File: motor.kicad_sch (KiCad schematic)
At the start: 20 parts, among them J201 JST-SH, J202 JST-SH, J203 JST-SH, J204 JST-SH, U201 A4950E, U202 A4950E, U203 A4950E, U204 A4950E

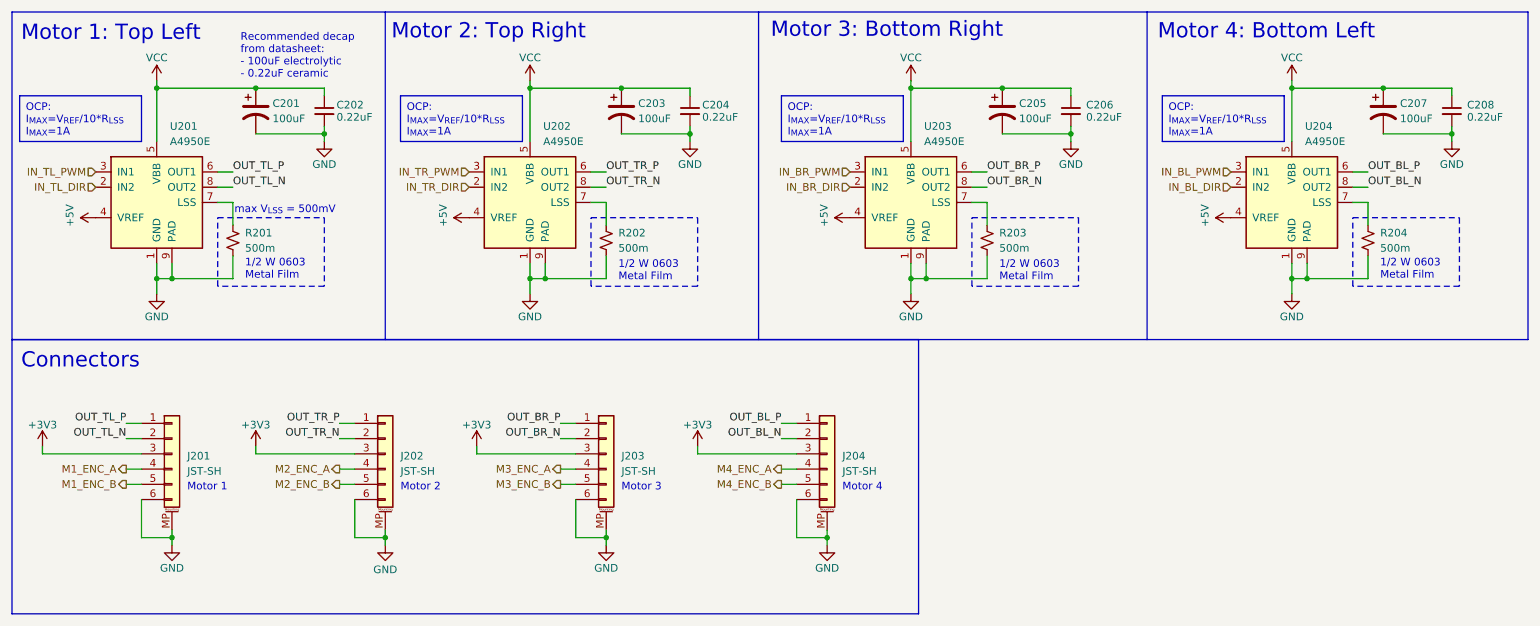
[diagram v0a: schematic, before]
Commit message: version 2 done
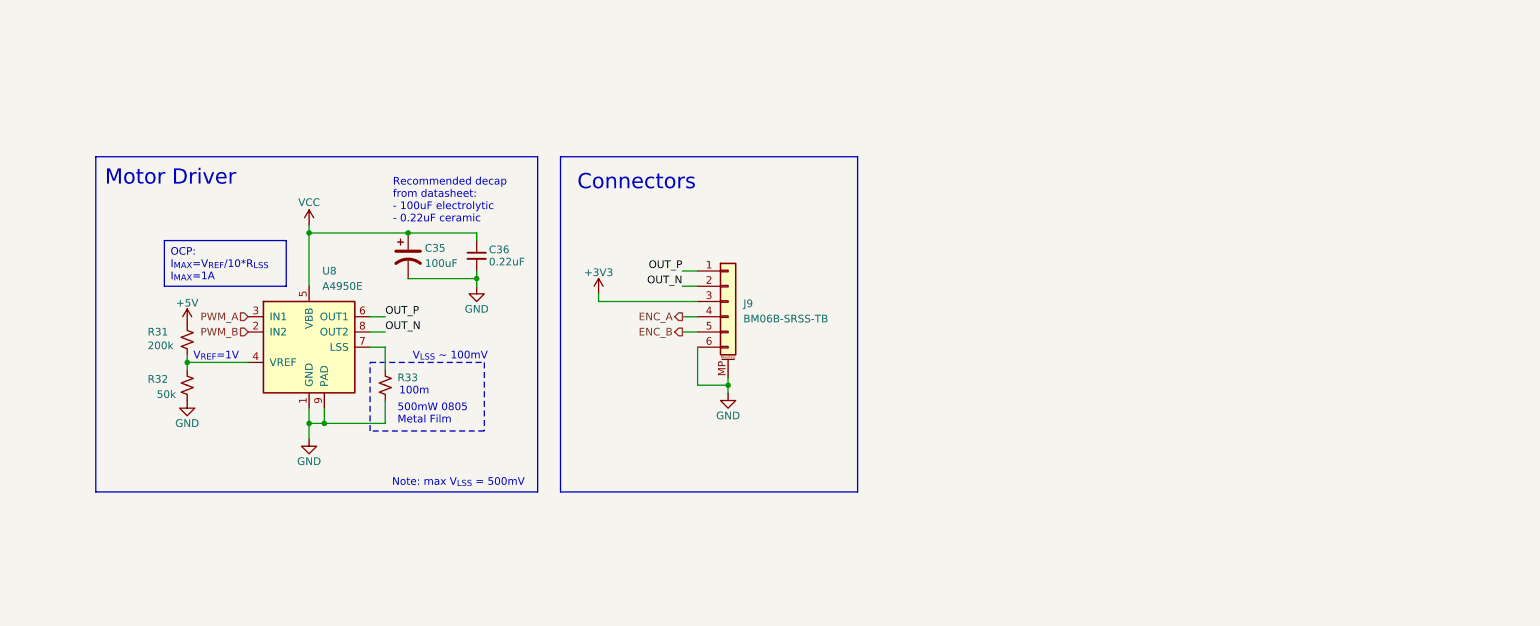
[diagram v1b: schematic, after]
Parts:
- removed C203, C205, C207: 100uF, Capacitor_SMD:CP_Elec_6.3x7.7, symbol Device:C_Polarized_US
- removed C204, C206, C208: 0.22uF, Capacitor_SMD:C_0603_1608Metric, symbol Device:C_Small
- removed J202, J203, J204: JST-SH, Connector_JST:JST_SH_SM06B-SRSS-TB_1x06-1MP_P1.00mm_Horizontal, symbol Connector_Generic_MountingPin:Conn_01x06_MountingPin
- removed R202, R203, R204: 500m, Resistor_SMD:R_0603_1608Metric, symbol Device:R_Small_US
- removed U202, U203, U204: A4950E, Package_SO:SOIC-8-1EP_3.9x4.9mm_P1.27mm_EP2.41x3.3mm_ThermalVias, symbol Driver_Motor:A4950E
- added R31: 200k, Resistor_SMD:R_0402_1005Metric, symbol Device:R_Small_US
- added R32: 50k, Resistor_SMD:R_0402_1005Metric, symbol Device:R_Small_US
- J9: renamed from J201; value JST-SH -> BM06B-SRSS-TB; footprint Connector_JST:JST_SH_SM06B-SRSS-TB_1x06-1MP_P1.00mm_Horizontal -> Connector_JST:JST_SH_BM06B-SRSS-TB_1x06-1MP_P1.00mm_Vertical
- R33: renamed from R201; value 500m -> RL10FTNR100; footprint Resistor_SMD:R_0603_1608Metric -> Resistor_SMD:R_0805_2012Metric
- renumbered C201 to C35, C202 to C36, U201 to U8
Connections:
- net +5V: now also R31.2; no longer U8.4 (VREF)
- net GND: now also R32.1
- net IN_TL_DIR renamed PWM_B
- net IN_TL_PWM renamed PWM_A
- net M1_ENC_A renamed ENC_A
- net M1_ENC_B renamed ENC_B
- net OUT_TL_N renamed OUT_N
- net OUT_TL_P renamed OUT_P
- new net: R31.1, R32.2, U8.4 (VREF)
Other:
- note added: "100m"
- note added: "500mW 0805 Metal Film"
- note added: "Motor Driver"
- note added: "Note: max V_{LSS} = 500mV"
- note added: "V_{LSS} ~ 100mV"
- note added: "V_{REF}=1V"
- note removed: "1/2 W 0603 Metal Film"
- note removed: "Motor 1"
- note removed: "Motor 1: Top Left"
- note removed: "Motor 2"
- note removed: "Motor 2: Top Right"
- note removed: "Motor 3"
- note removed: "Motor 3: Bottom Right"
- note removed: "Motor 4"
- note removed: "Motor 4: Bottom Left"
- note removed: "max V_{LSS} = 500mV"
- moved on the sheet: C35, C36, J9, R33, U8
